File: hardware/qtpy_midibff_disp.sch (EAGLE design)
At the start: 9 parts, among them J1 SJ-3523-SMT, J2 SJ-3523-SMT, U1 ADAFRUIT_QTPYM0, U2 6N137

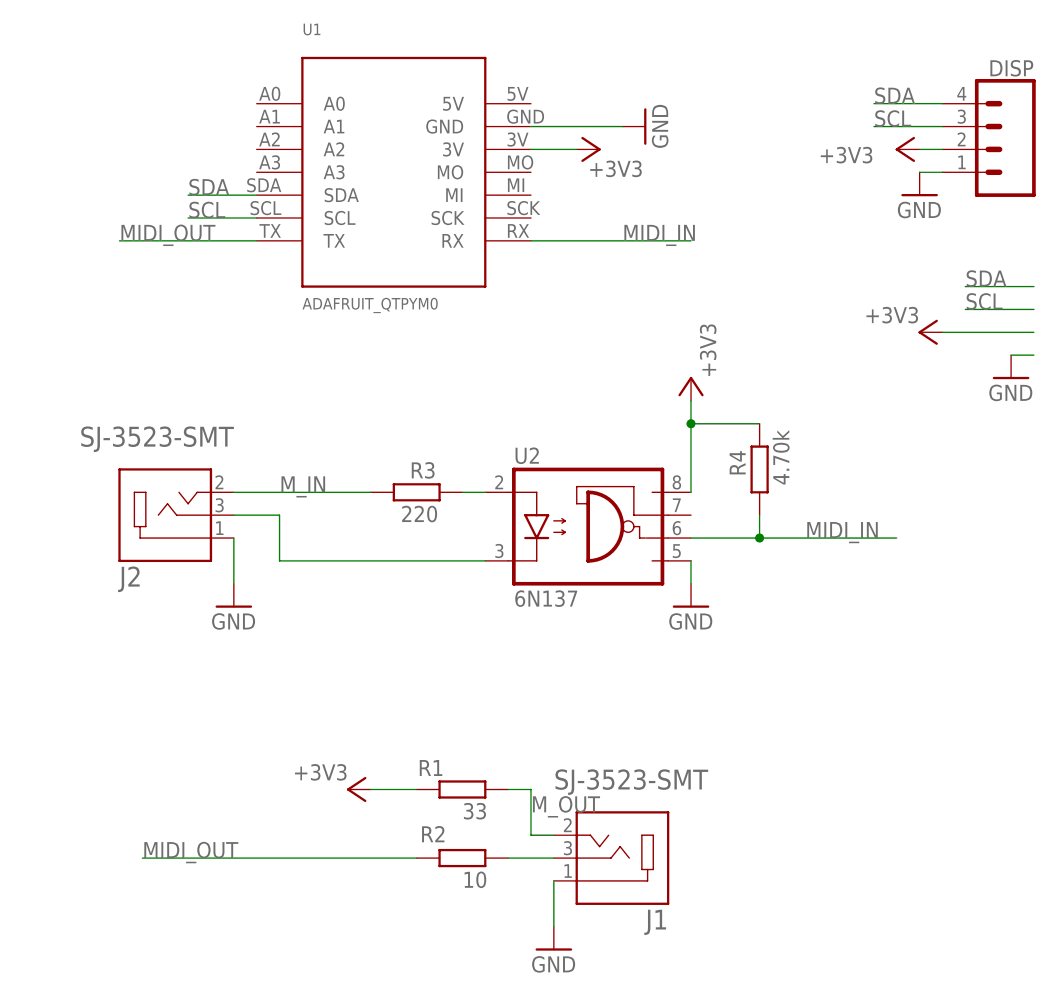
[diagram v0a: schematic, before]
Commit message: sigh trs-a/b will kill me
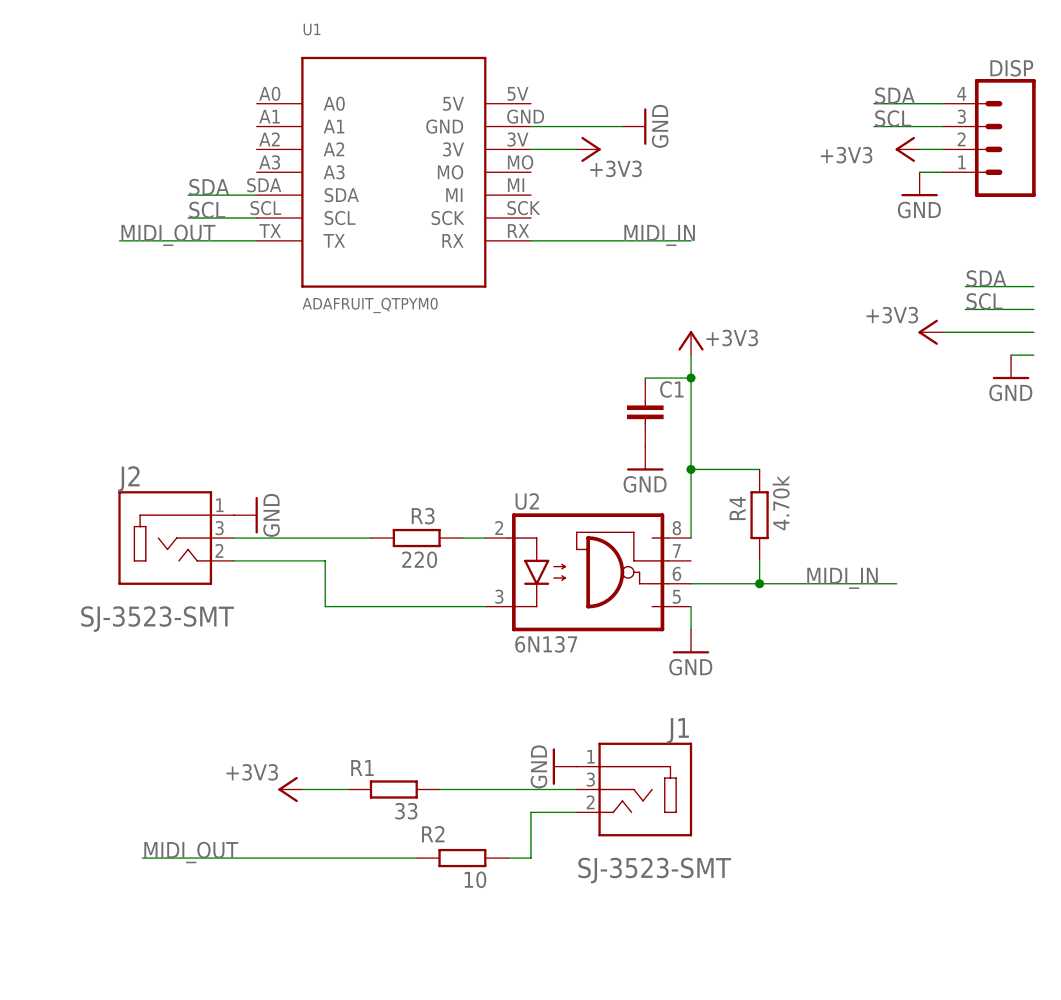
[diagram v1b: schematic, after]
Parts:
- added C1: (no value), rcl:C-EU025-025X050
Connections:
- removed net M_IN: J2.2, R3.2
- removed net M_OUT: J1.2, R1.1
- new net N$3: J2.2, U2.C
- new net N$5: J1.2, R2.1
- net +3V3: now also C1.1
- net GND: now also C1.2
- net N$1: now also R1.1; no longer R2.1
- net N$4: now also R3.2; no longer U2.C
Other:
- moved on the sheet: J1, J2, R1, R3, R4, U2
